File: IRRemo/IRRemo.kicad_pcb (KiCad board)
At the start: 2 copper layers, 48.3 x 33 mm, 16 parts, among them J1 Conn_01x05_Male, J2 Conn_02x02_Odd_Even, J3 Conn_01x03_Male, J4 Conn_01x02_Male, J5 Conn_01x02_Male, U1 CY8C4244, U2 GP1UXC41QS, U3 BD6211F, U4 BD6211F

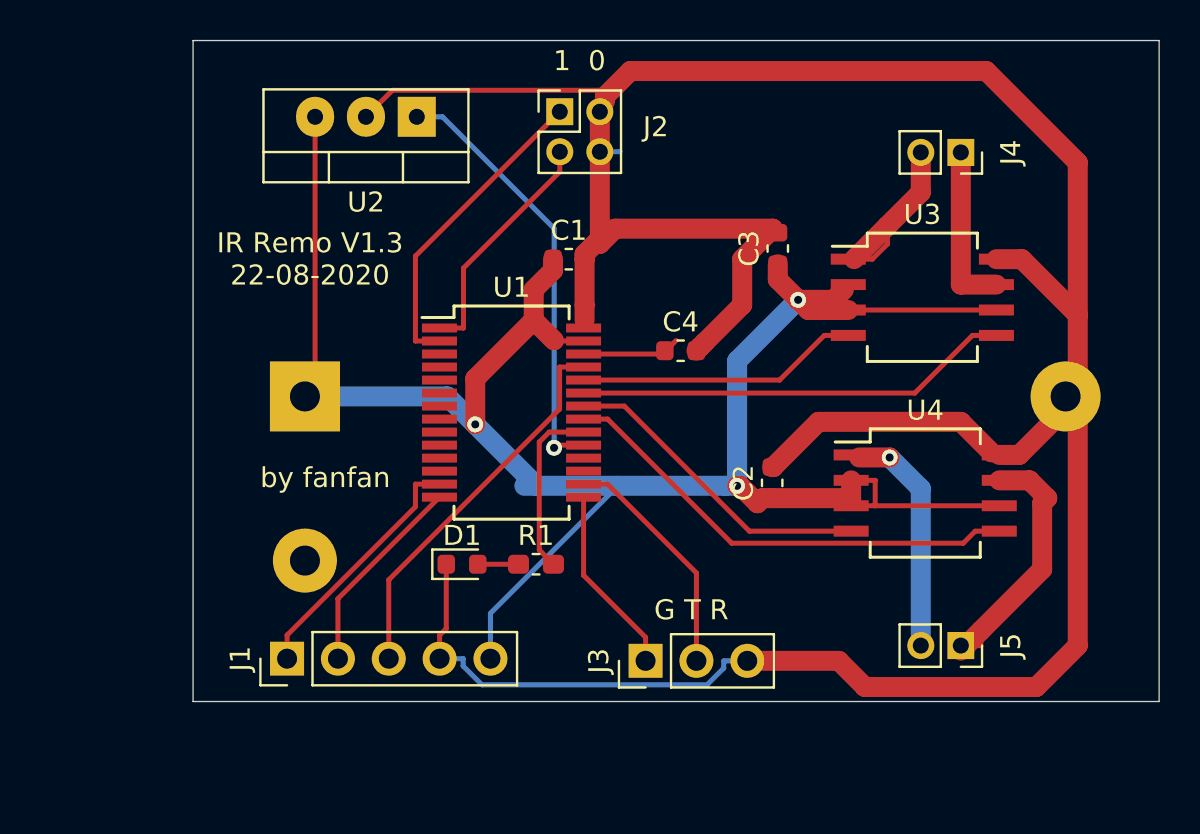
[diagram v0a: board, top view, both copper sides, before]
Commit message: BGA
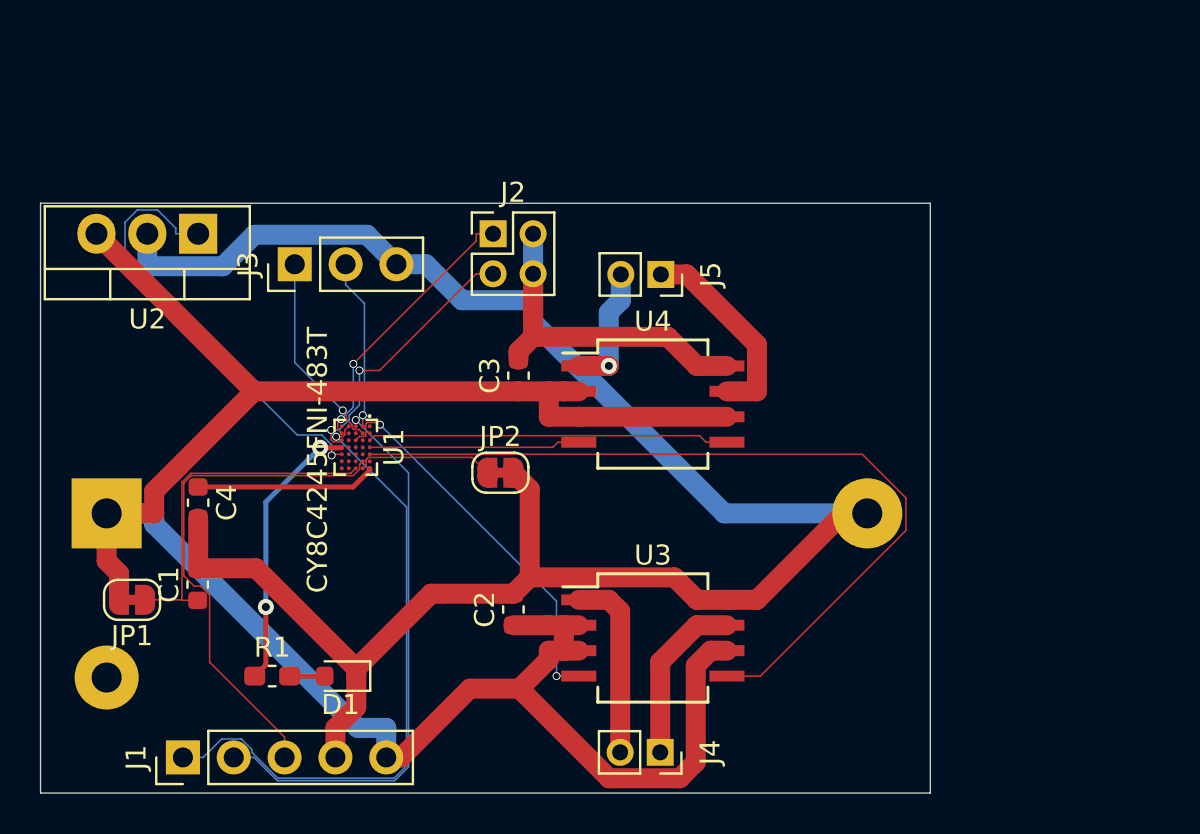
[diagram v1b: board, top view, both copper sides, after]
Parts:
- added JP1: SolderJumper_2_Bridged, 2020-08-21_07-11-41:Jumper-Con, F.Cu at (90.9, 96.5)
- added JP2: SolderJumper_2_Bridged, 2020-08-21_07-11-41:Jumper-Con, F.Cu at (109.3, 90.2)
- J2: value Conn_02x02_Odd_Even -> SER
- U1: value CY8C4244 -> CY8C4245FNI-483T; footprint Package_SO:SSOP-28_5.3x10.2mm_P0.65mm -> 2020-08-21_07-11-41:BGA35N35P7X5_258X209X48N
- moved J4 33.5 mm to (117.3, 104.1)
- moved J3 26.5 mm to (99.1, 79.8)
- moved C4 25.3 mm to (94.2, 91.7), turned to 270 degrees
- moved C1 24.7 mm to (94.2, 95.8), turned to 90 degrees
- moved J5 23.8 mm to (117.3, 80.3)
- moved U3 21.7 mm to (117.0, 98.4)
- moved C3 14.4 mm to (110.2, 85.3)
- moved C2 14.4 mm to (110.0, 97.0)
- moved R1 14.3 mm to (97.9, 100.3)
- moved U4 14.3 mm to (117.0, 86.7)
- moved U2 12.4 mm to (94.2, 78.2)
- moved BT1 11.5 mm to (89.7, 92.2)
- moved D1 8.25 mm to (101.3, 100.3), turned to 180 degrees
- moved U1 7.97 mm to (102.1, 88.9), turned to 270 degrees
- moved J1 7.17 mm to (93.5, 104.4)
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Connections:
- C1 pad 1: +3V0 -> VDD
- R1 pad 1: Net-(D1-Pad2) -> Net-(R1-Pad1)
- R1 pad 2: Net-(R1-Pad2) -> Net-(D1-Pad2)
- U3 pad 4: Net-(U1-Pad24) -> Net-(U1-PadC3)
- U3 pad 5: Net-(U1-Pad23) -> Net-(U1-PadA5)
- U4 pad 4: Net-(U1-Pad22) -> Net-(U1-PadA4)
- U4 pad 5: Net-(U1-Pad21) -> Net-(U1-PadA3)
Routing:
- net GND: track 159.7 -> 115.5 mm
- net Net-(U1-PadA5): track 0.00 -> 41.3 mm
- net Net-(U1-Pad21): track 23.6 -> 0.00 mm
- net Net-(U1-Pad23): track 21.8 -> 0.00 mm
- net Net-(U1-PadC3): track 0.00 -> 19.3 mm, vias 0 -> 2
- net SWDIO: track 12.6 -> 31.6 mm, vias 0 -> 1
- net Net-(U1-PadA3): track 0.00 -> 18.1 mm
- net SWDCK: track 10.2 -> 28.2 mm, vias 0 -> 1
- net VDD: track 0.00 -> 17.5 mm
- net Net-(U1-Pad22): track 16.0 -> 0.00 mm
- net Net-(U1-Pad24): track 14.1 -> 0.00 mm
- net Net-(R1-Pad1): track 0.00 -> 13.9 mm, vias 0 -> 2
- net Net-(U1-PadA4): track 0.00 -> 10.5 mm
- net Net-(R1-Pad2): track 8.82 -> 0.00 mm
- net Vss: track 0.00 -> 6.92 mm
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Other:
- board size 48.3 x 33 mm -> 44.5 x 29.5 mm
- net class BGA added: clearance 0.01, trace_width 0.08, via_dia 0.4, via_drill 0.3
- net class Default: clearance 0.2 -> 0.05
- net class Pow added: clearance 0.12, trace_width 1, via_dia 0.8, via_drill 0.4
- rule solder_mask_min_width: 0.25 -> 0.1
- rule trace_clearance: 0.2 -> 0.05
- rule trace_min: 0.2 -> 0.08
- rule via_min_drill: 0.3 -> 0.2
- rule via_min_size: 0.4 -> 0.3
- board text removed: "1 0"
- board text removed: "G T R"
- board text removed: "IR Remo V1.3 22-08-2020"
- board text removed: "by fanfan"
